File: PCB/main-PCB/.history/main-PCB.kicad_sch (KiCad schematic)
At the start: 25 parts, among them Q1 SSM6J214FE, Q2 Q_NMOS_GSD, U1 LIS2DU12TR, U2 STM32U031K4Ux

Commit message: -Updated MCU part number -Changed to 0402 passives
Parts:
- C2, C3, C5, C6, C7: footprint Capacitor_SMD:C_0402_1005Metric -> Capacitor_SMD:C_0201_0603Metric
- R1, R2, R3, R4: footprint Resistor_SMD:R_0402_1005Metric -> Resistor_SMD:R_0201_0603Metric
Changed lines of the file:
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@@
 			)
 		)
-		(property "Footprint" "Capacitor_SMD:C_0402_1005Metric"
+		(property "Footprint" "Capacitor_SMD:C_0201_0603Metric"
 			(at 56.1848 130.81 0)
 			(hide yes)
@@
 			)
 		)
-		(property "Footprint" "Capacitor_SMD:C_0402_1005Metric"
+		(property "Footprint" "Capacitor_SMD:C_0201_0603Metric"
 			(at 147.6248 72.39 0)
 			(hide yes)
@@
 			)
 		)
-		(property "Footprint" "Capacitor_SMD:C_0402_1005Metric"
+		(property "Footprint" "Capacitor_SMD:C_0201_0603Metric"
 			(at 134.9248 72.39 0)
 			(hide yes)
@@
 			)
 		)
-		(property "Footprint" "Resistor_SMD:R_0402_1005Metric"
+		(property "Footprint" "Resistor_SMD:R_0201_0603Metric"
 			(at 83.312 60.96 90)
 			(hide yes)
@@
 			)
 		)
-		(property "Footprint" "Resistor_SMD:R_0402_1005Metric"
+		(property "Footprint" "Resistor_SMD:R_0201_0603Metric"
 			(at 239.522 114.3 90)
 			(hide yes)
@@
 			)
 		)
-		(property "Footprint" "Capacitor_SMD:C_0402_1005Metric"
+		(property "Footprint" "Capacitor_SMD:C_0201_0603Metric"
 			(at 163.5252 72.39 0)
 			(hide yes)
@@
 			)
 		)
-		(property "Footprint" "Capacitor_SMD:C_0402_1005Metric"
+		(property "Footprint" "Capacitor_SMD:C_0201_0603Metric"
 			(at 56.1848 109.22 0)
 			(hide yes)
@@
 			)
 		)
-		(property "Footprint" "Resistor_SMD:R_0402_1005Metric"
+		(property "Footprint" "Resistor_SMD:R_0201_0603Metric"
 			(at 260.858 83.82 90)
 			(hide yes)
@@
 			)
 		)
-		(property "Footprint" "Resistor_SMD:R_0402_1005Metric"
+		(property "Footprint" "Resistor_SMD:R_0201_0603Metric"
 			(at 248.158 83.82 90)
 			(hide yes)

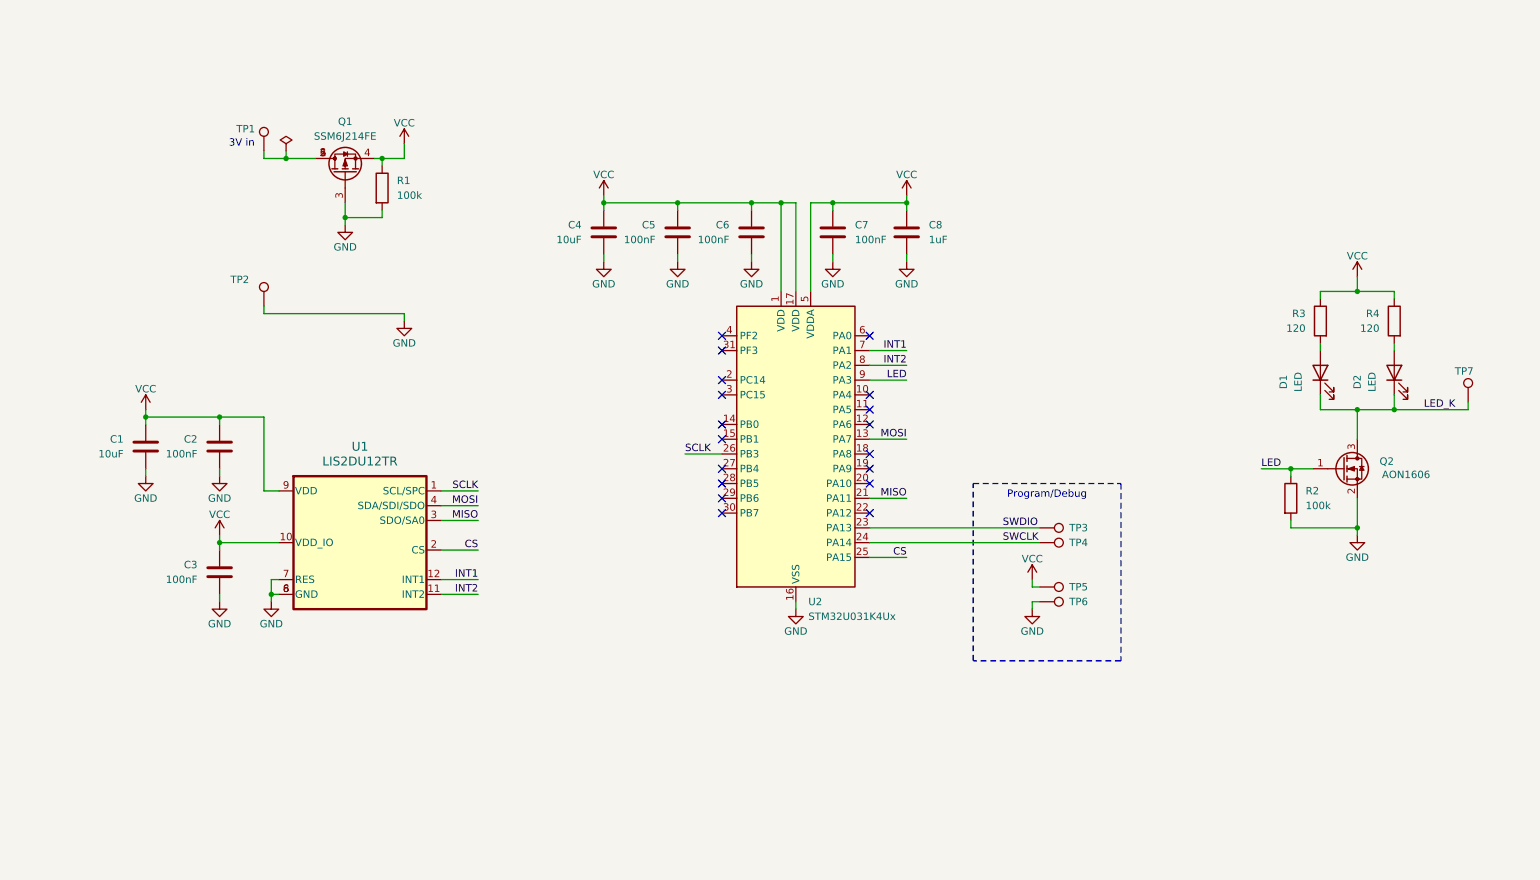
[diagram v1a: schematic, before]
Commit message: Updated PCB STEP file
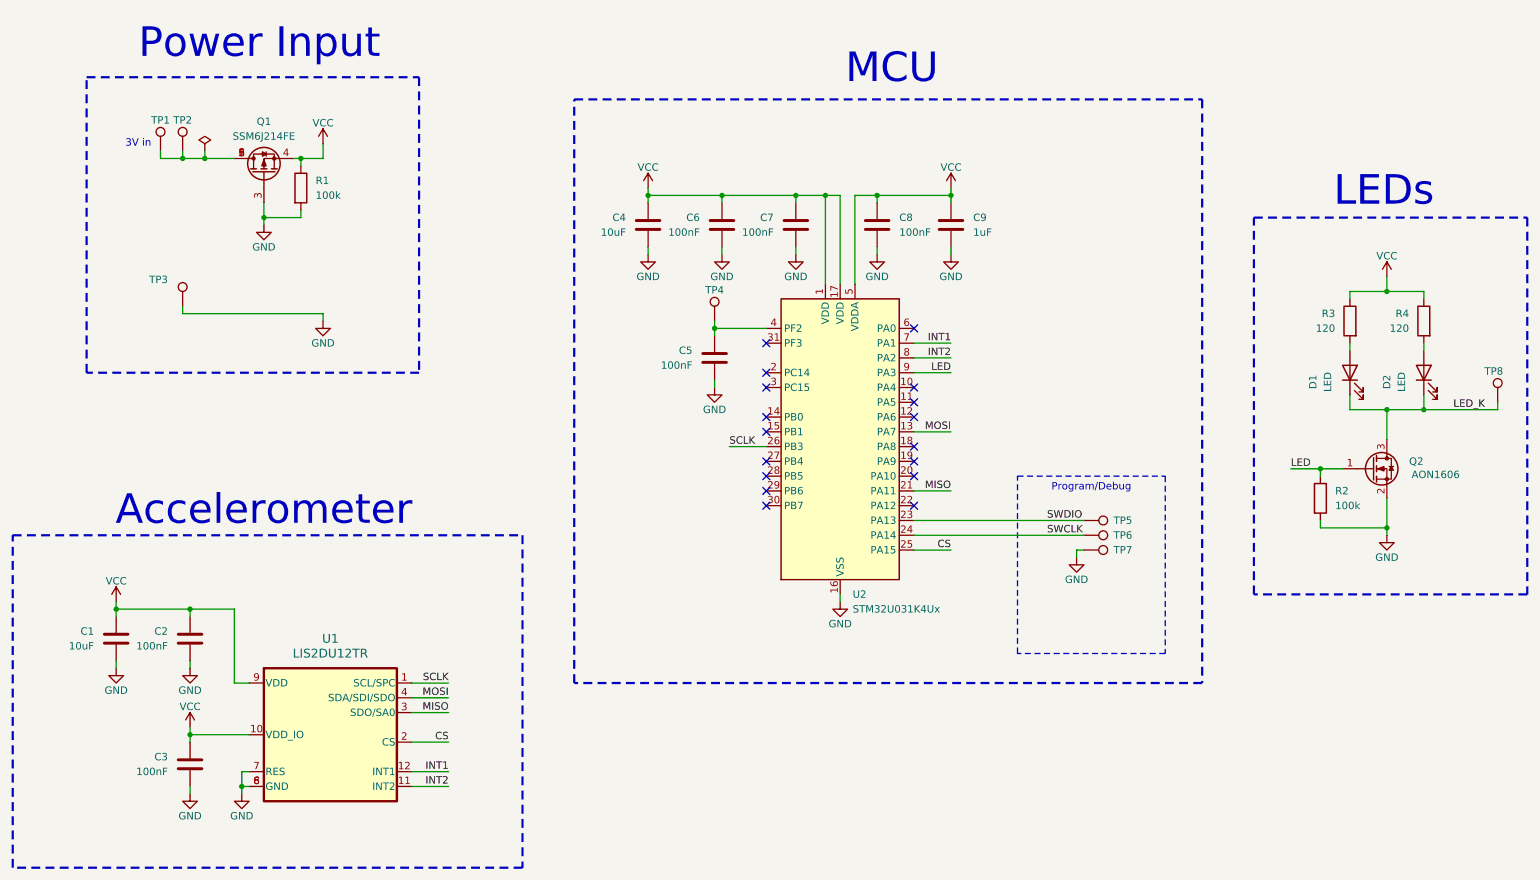
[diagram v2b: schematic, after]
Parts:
- removed TP5: TestPoint, TestPoint:TestPoint_Pad_D1.0mm, symbol Connector:TestPoint
- added C5: 100nF, Capacitor_SMD:C_0402_1005Metric, symbol Device:C
- added TP2: TestPoint, TestPoint:TestPoint_Pad_D1.0mm, symbol Connector:TestPoint
- added TP4: TestPoint, EN_Designs-Footprints:TestPoint_Pad_D0.5mm, symbol Connector:TestPoint
- C2, C3: footprint Capacitor_SMD:C_0201_0603Metric -> Capacitor_SMD:C_0402_1005Metric
- C6: renamed from C5; footprint Capacitor_SMD:C_0201_0603Metric -> Capacitor_SMD:C_0402_1005Metric
- C7: renamed from C6; footprint Capacitor_SMD:C_0201_0603Metric -> Capacitor_SMD:C_0402_1005Metric
- C8: renamed from C7; footprint Capacitor_SMD:C_0201_0603Metric -> Capacitor_SMD:C_0402_1005Metric
- R1, R2, R3, R4: footprint Resistor_SMD:R_0201_0603Metric -> Resistor_SMD:R_0402_1005Metric
- TP5: renamed from TP3; now left out of the parts list
- TP6: renamed from TP4; now left out of the parts list
- TP7: renamed from TP6; now left out of the parts list
- U2: MPN (none) -> STM32U031K4U6
- renumbered C8 to C9, TP2 to TP3, TP7 to TP8
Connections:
- net GND: now also C5.2
- net at Q1.1 (D), Q1.2 (D), Q1.5 (D)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: now also TP2.1
- net at U2.4 (PF2): now also C5.1, TP4.1
- no-connect marks 18 -> 17
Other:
- note added: "Accelerometer"
- note added: "LEDs"
- note added: "MCU"
- note added: "Power Input"
- moved on the sheet: C1, C2, C3, C4, C6, C7, C8, C9, D1, D2, Q1, Q2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
